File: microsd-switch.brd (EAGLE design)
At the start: 49.2 x 41.9 mm, 12 parts, among them IC1 SN74CBT3257D, IC2 SN74CBT3257D, U1 USD-SOCKETNEW

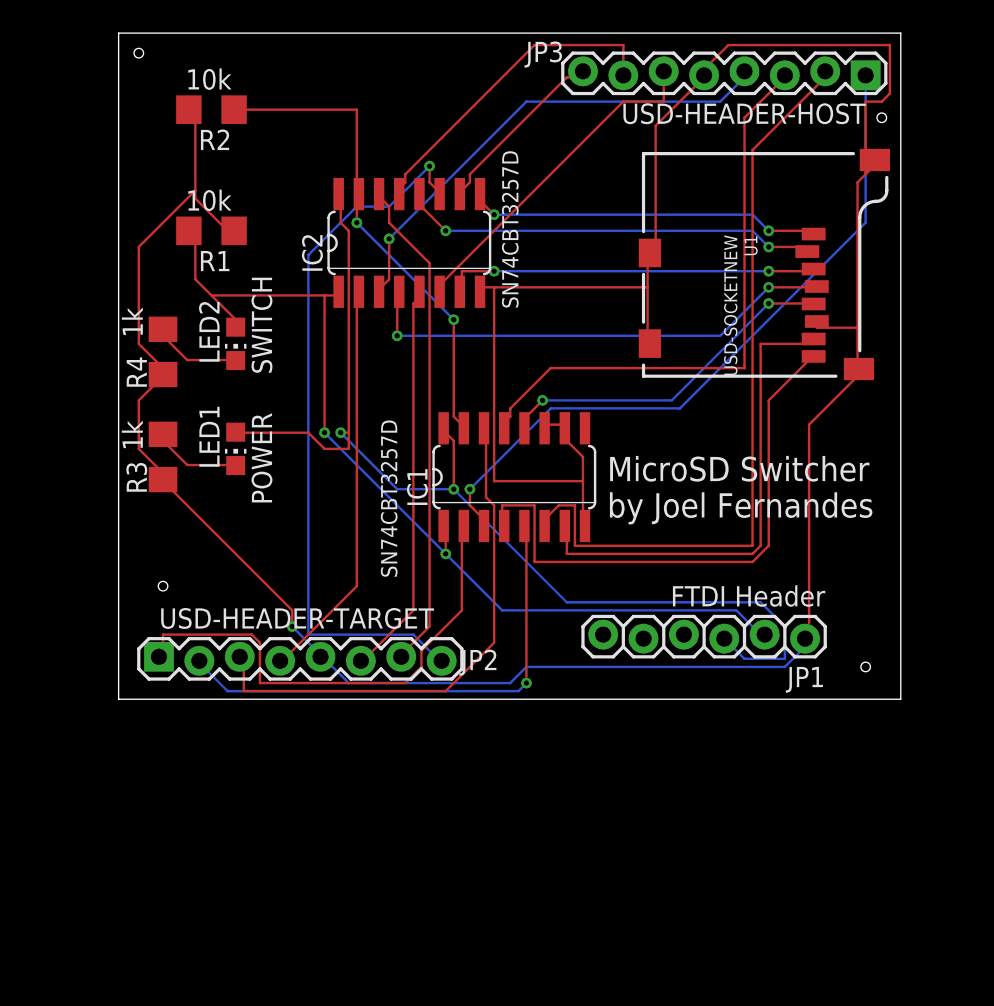
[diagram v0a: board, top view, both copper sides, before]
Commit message: MicroSD Switch Rev Alpha released
Signed-off-by: Joel Fernandes <joelf@ti.com>
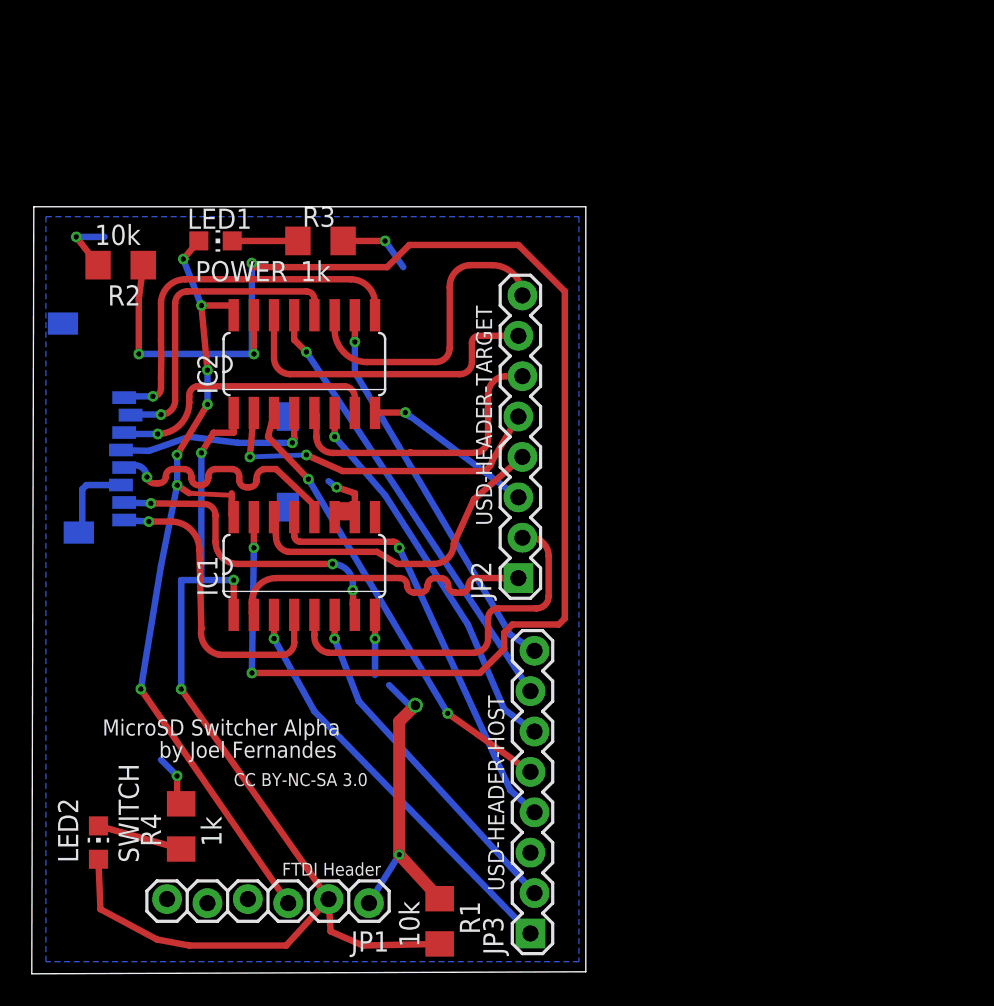
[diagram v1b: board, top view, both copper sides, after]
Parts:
- moved JP3 58.0 mm to (60.3, 23.4), turned to 90 degrees
- moved R1 45.7 mm to (54.5, 24.1), turned to 270 degrees
- moved LED2 32.5 mm to (33.0, 29.1), turned to 0 degrees
- moved JP1 32.1 mm to (50.0, 25.3)
- moved R4 29.9 mm to (38.2, 30.1), turned to 90 degrees
- moved U1 24.3 mm to (45.3, 48.1), flipped to the bottom
- moved JP2 23.3 mm to (59.6, 45.7), turned to 90 degrees
- moved R3 16.8 mm to (47.0, 66.9), turned to 0 degrees
- moved IC1 14.3 mm to (46.0, 46.5)
- moved LED1 13.1 mm to (40.4, 66.9), turned to 270 degrees
- moved R2 11.3 mm to (34.4, 65.4)
- moved IC2 10.1 mm to (46.0, 59.2)
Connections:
- net N$1 renamed CLK-Y
- net CLK-A: now also JP2.4; no longer JP2.3
- net CLK-B: now also JP3.4; no longer JP3.3
- net GND: now also JP2.3, JP3.3; no longer JP2.5, JP3.5
- net VDD-A: now also JP2.5; no longer JP2.4
- net VDD-B: now also JP3.5; no longer JP3.4
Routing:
- net GND: track 191.6 -> 61.4 mm, vias 1 -> 8
- net OE: track 30.6 -> 94.8 mm, vias 2 -> 5
- net DAT0-B: track 48.2 -> 22.1 mm, vias 0 -> 1
- net DAT2-A: track 44.8 -> 19.1 mm, vias 1 -> 0
- net DAT1-B: track 43.9 -> 26.2 mm
- net N$2: track 30.5 -> 12.9 mm, vias 2 -> 1
- net DAT1-Y: track 35.2 -> 19.2 mm, vias 0 -> 1
- net VCC: track 67.8 -> 53.6 mm, vias 2 -> 7
- net DAT2-B: track 11.5 -> 24.6 mm, vias 0 -> 1
- net CLK-A: track 33.1 -> 20.7 mm
- net DAT1-A: track 30.9 -> 19.8 mm
- net DAT0-Y: track 30.4 -> 19.4 mm, vias 0 -> 3
- net DAT3-A: track 31.1 -> 20.2 mm
- net CLK-B: track 36.7 -> 26.9 mm, vias 0 -> 1
- net HOSTSELECT: track 59.3 -> 68.9 mm, vias 2 -> 3
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- added copper zone on layer 16, net GND
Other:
- board size 49.2 x 41.9 mm -> 34.8 x 48.2 mm
- board text added: "CC BY-NC-SA 3.0"
- board text added: "MicroSD Switcher Alpha"
- board text added: "by Joel Fernandes"
- board text removed: "MicroSD Switcher by Joel Fernandes"
